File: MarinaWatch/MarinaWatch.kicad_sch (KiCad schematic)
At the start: 14 parts, among them J1 USB_C_Receptacle_USB2.0_16P, U1 ESP32-S3-WROOM-1, U3 BQ24166RGE

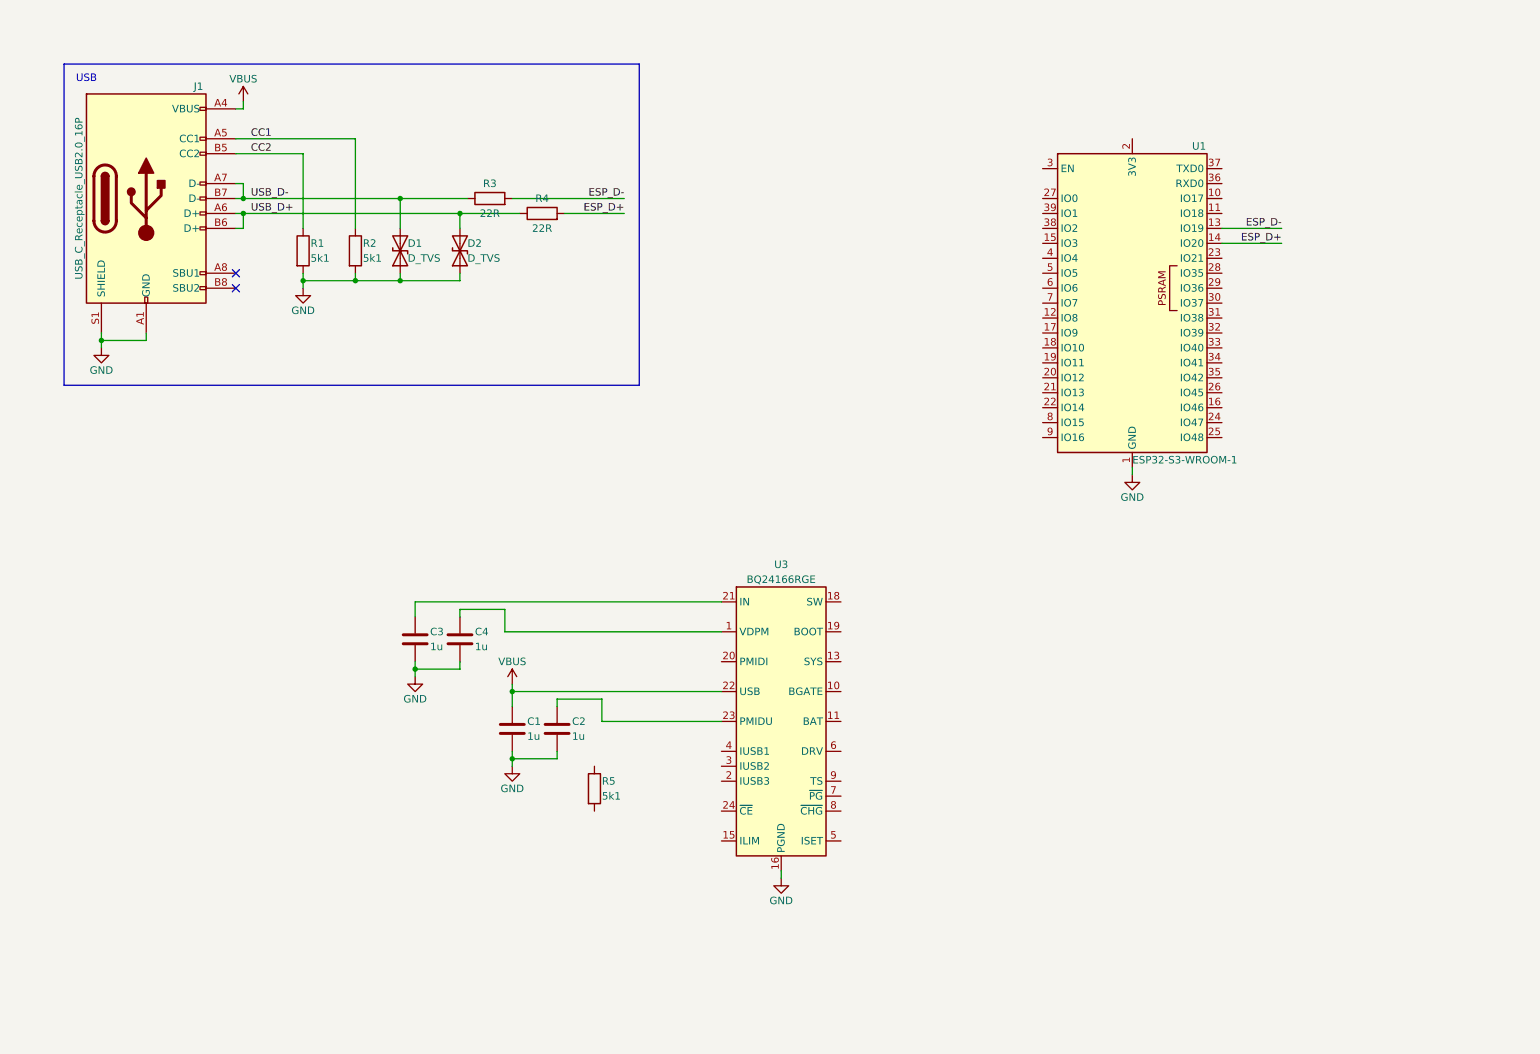
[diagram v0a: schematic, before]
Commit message: Structure power supply chain
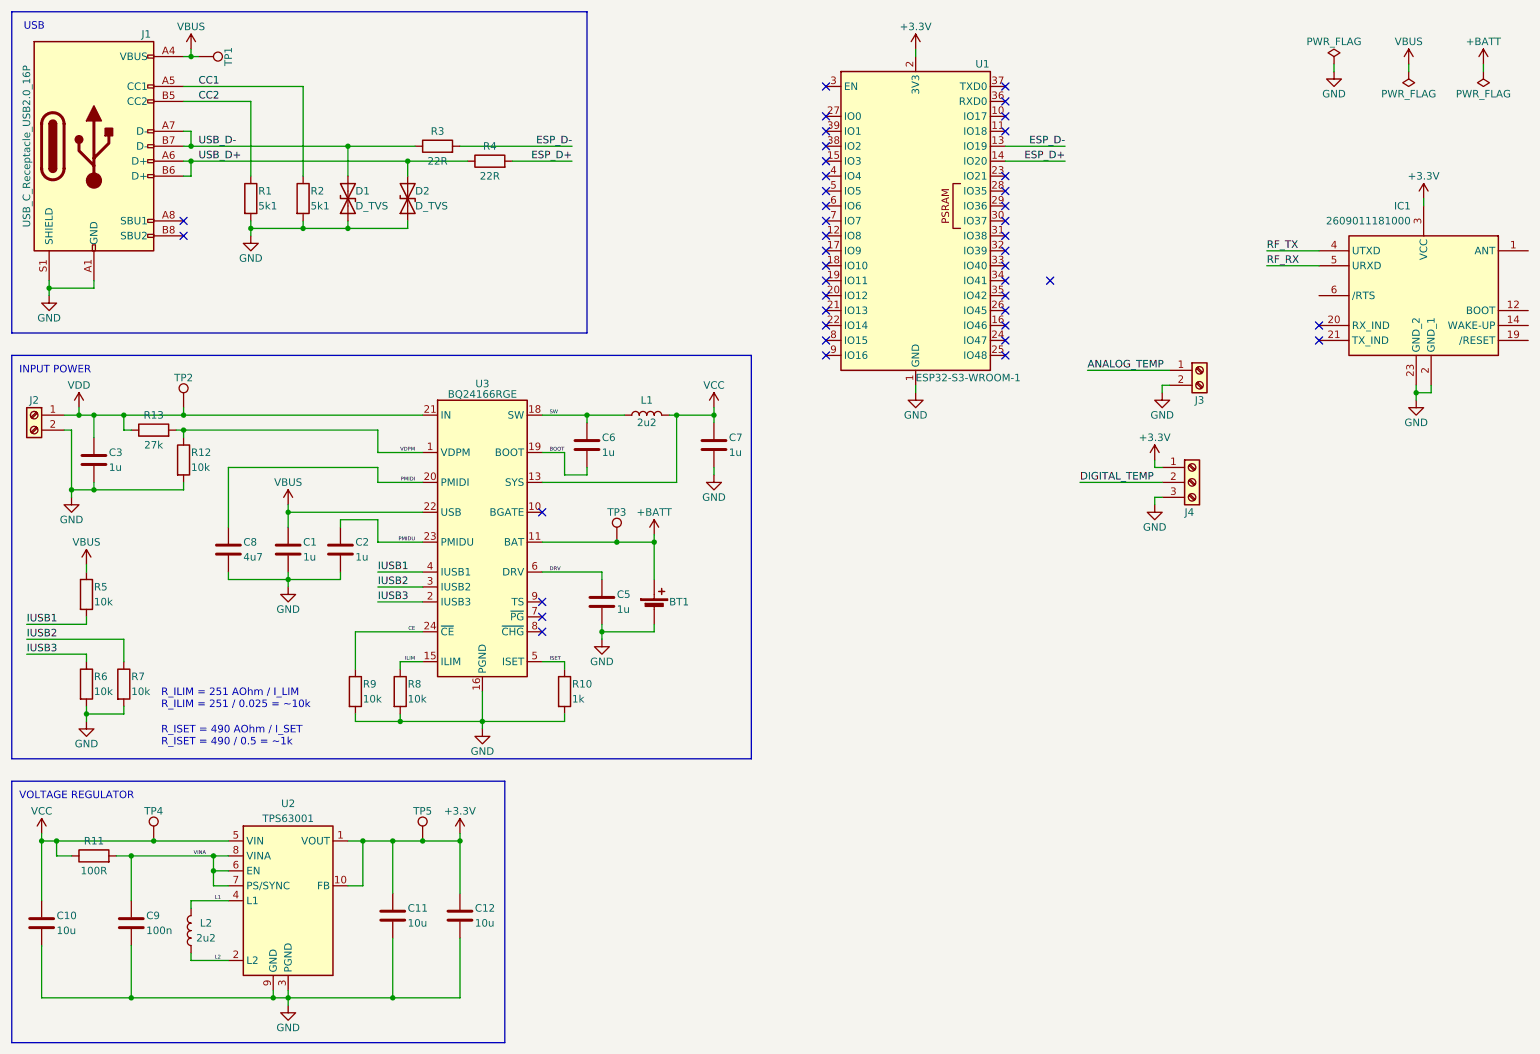
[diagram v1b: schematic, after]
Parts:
- removed C4: 1u, Capacitor_SMD:C_0603_1608Metric_Pad1.08x0.95mm_HandSolder, symbol Device:C
- added BT1: Battery_Cell, symbol Device:Battery_Cell
- added C10, C11, C12: 10u, Capacitor_SMD:C_0603_1608Metric_Pad1.08x0.95mm_HandSolder, symbol Device:C
- added C5, C6, C7: 1u, Capacitor_SMD:C_0603_1608Metric_Pad1.08x0.95mm_HandSolder, symbol Device:C
- added C8: 4u7, Capacitor_SMD:C_0603_1608Metric_Pad1.08x0.95mm_HandSolder, symbol Device:C
- added C9: 100n, Capacitor_SMD:C_0603_1608Metric_Pad1.08x0.95mm_HandSolder, symbol Device:C
- added IC1: 2609011181000, Lund Formula Student:2609011181000, symbol Lund Formula Student:2609011181000
- added J2: Screw_Terminal_01x02, TerminalBlock_Phoenix:TerminalBlock_Phoenix_MKDS-3-2-5.08_1x02_P5.08mm_Horizontal, symbol Connector:Screw_Terminal_01x02
- added J3: Screw_Terminal_01x02, symbol Connector:Screw_Terminal_01x02
- added J4: Screw_Terminal_01x03, symbol Connector:Screw_Terminal_01x03
- added L1, L2: 2u2, Inductor_SMD_Wurth:L_Wurth_WE-LQSH-4020, symbol Device:L
- added R10: 1k, Resistor_SMD:R_0603_1608Metric_Pad0.98x0.95mm_HandSolder, symbol Device:R
- added R11: 100R, Resistor_SMD:R_0603_1608Metric_Pad0.98x0.95mm_HandSolder, symbol Device:R
- added R12, R6, R7, R8, R9: 10k, Resistor_SMD:R_0603_1608Metric_Pad0.98x0.95mm_HandSolder, symbol Device:R
- added R13: 27k, Resistor_SMD:R_0603_1608Metric_Pad0.98x0.95mm_HandSolder, symbol Device:R
- added TP1, TP2, TP3, TP4, TP5: TestPoint, TestPoint:TestPoint_Pad_D2.0mm, symbol Connector:TestPoint
- added U2: TPS63001, Package_SON:Texas_DRC0010J_ThermalVias, symbol Regulator_Switching:TPS63001
- R5: value 5k1 -> 10k
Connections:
- net GND: now also BT1.2 (-), C10.2, C11.2, C12.2, C5.2, C7.2, C8.2, C9.2, IC1.2 (GND_1), IC1.23 (GND_2), J2.2 (Pin_2), J3.2 (Pin_2), J4.3 (Pin_3), R10.2, R12.2, R6.2, R7.2, R8.2, R9.2, U2.11 (PGND), U2.3 (PGND), U2.9 (GND)
- net VBUS: now also R5.1, TP1.1
- net IUSB1: now reaches R5.2
- net IUSB1: now also U3.4 (IUSB1)
- net VDPM: now reaches U3.1 (VDPM)
- net VDPM: now also R12.1, R13.2
- net +BATT: now reaches U3.11 (BAT), U3.12 (BAT)
- net +BATT: now also BT1.1 (+), TP3.1
- net VCC: now reaches U3.13 (SYS), U3.14 (SYS)
- net VCC: now also C10.1, C7.1, L1.2, R11.1, TP4.1, U2.5 (VIN)
- net ILIM: now reaches U3.15 (ILIM)
- net ILIM: now also R8.1
- net SW: now reaches U3.18 (SW)
- net SW: now also C6.1, L1.1
- net BOOT: now reaches U3.19 (BOOT)
- net BOOT: now also C6.2
- net IUSB3: now reaches U3.2 (IUSB3)
- net IUSB3: now also R6.1
- net PMIDI: now reaches U3.20 (PMIDI)
- net PMIDI: now also C8.1
- net VDD: now reaches C3.1, U3.21 (IN)
- net VDD: now also J2.1 (Pin_1), R13.1, TP2.1
- net PMIDU: now reaches C2.1, U3.23 (PMIDU)
- net CE: now reaches U3.24 (~{CE})
- net CE: now also R9.1
- net IUSB2: now reaches U3.3 (IUSB2)
- net IUSB2: now also R7.1
- net ISET: now reaches U3.5 (ISET)
- net ISET: now also R10.1
- net DRV: now reaches U3.6 (DRV)
- net DRV: now also C5.1
- net +3.3V: now reaches U1.2 (3V3)
- net +3.3V: now also C11.1, C12.1, IC1.3 (VCC), J4.1 (Pin_1), TP5.1, U2.1 (VOUT), U2.10 (FB)
- new net ANALOG_TEMP: J3.1 (Pin_1)
- new net DIGITAL_TEMP: J4.2 (Pin_2)
- new net L1: L2.2, U2.4 (L1)
- new net L2: L2.1, U2.2 (L2)
- new net RF_RX: IC1.5 (URXD)
- new net RF_TX: IC1.4 (UTXD)
- new net VINA: C9.1, R11.2, U2.6 (EN), U2.7 (PS/SYNC), U2.8 (VINA)
- no-connect marks 2 -> 44
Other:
- note added: "INPUT POWER"
- note added: "R_ILIM = 251 AOhm / I_LIM R_ILIM = 251 / 0.025 = ~10k"
- note added: "R_ISET = 490 AOhm / I_SET R_ISET = 490 / 0.5 = ~1k"
- note added: "VOLTAGE REGULATOR"
- moved on the sheet: C1, C2, C3, D1, D2, J1, R1, R2, R3, R4, U1, U3
